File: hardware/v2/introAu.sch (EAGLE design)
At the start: 24 parts

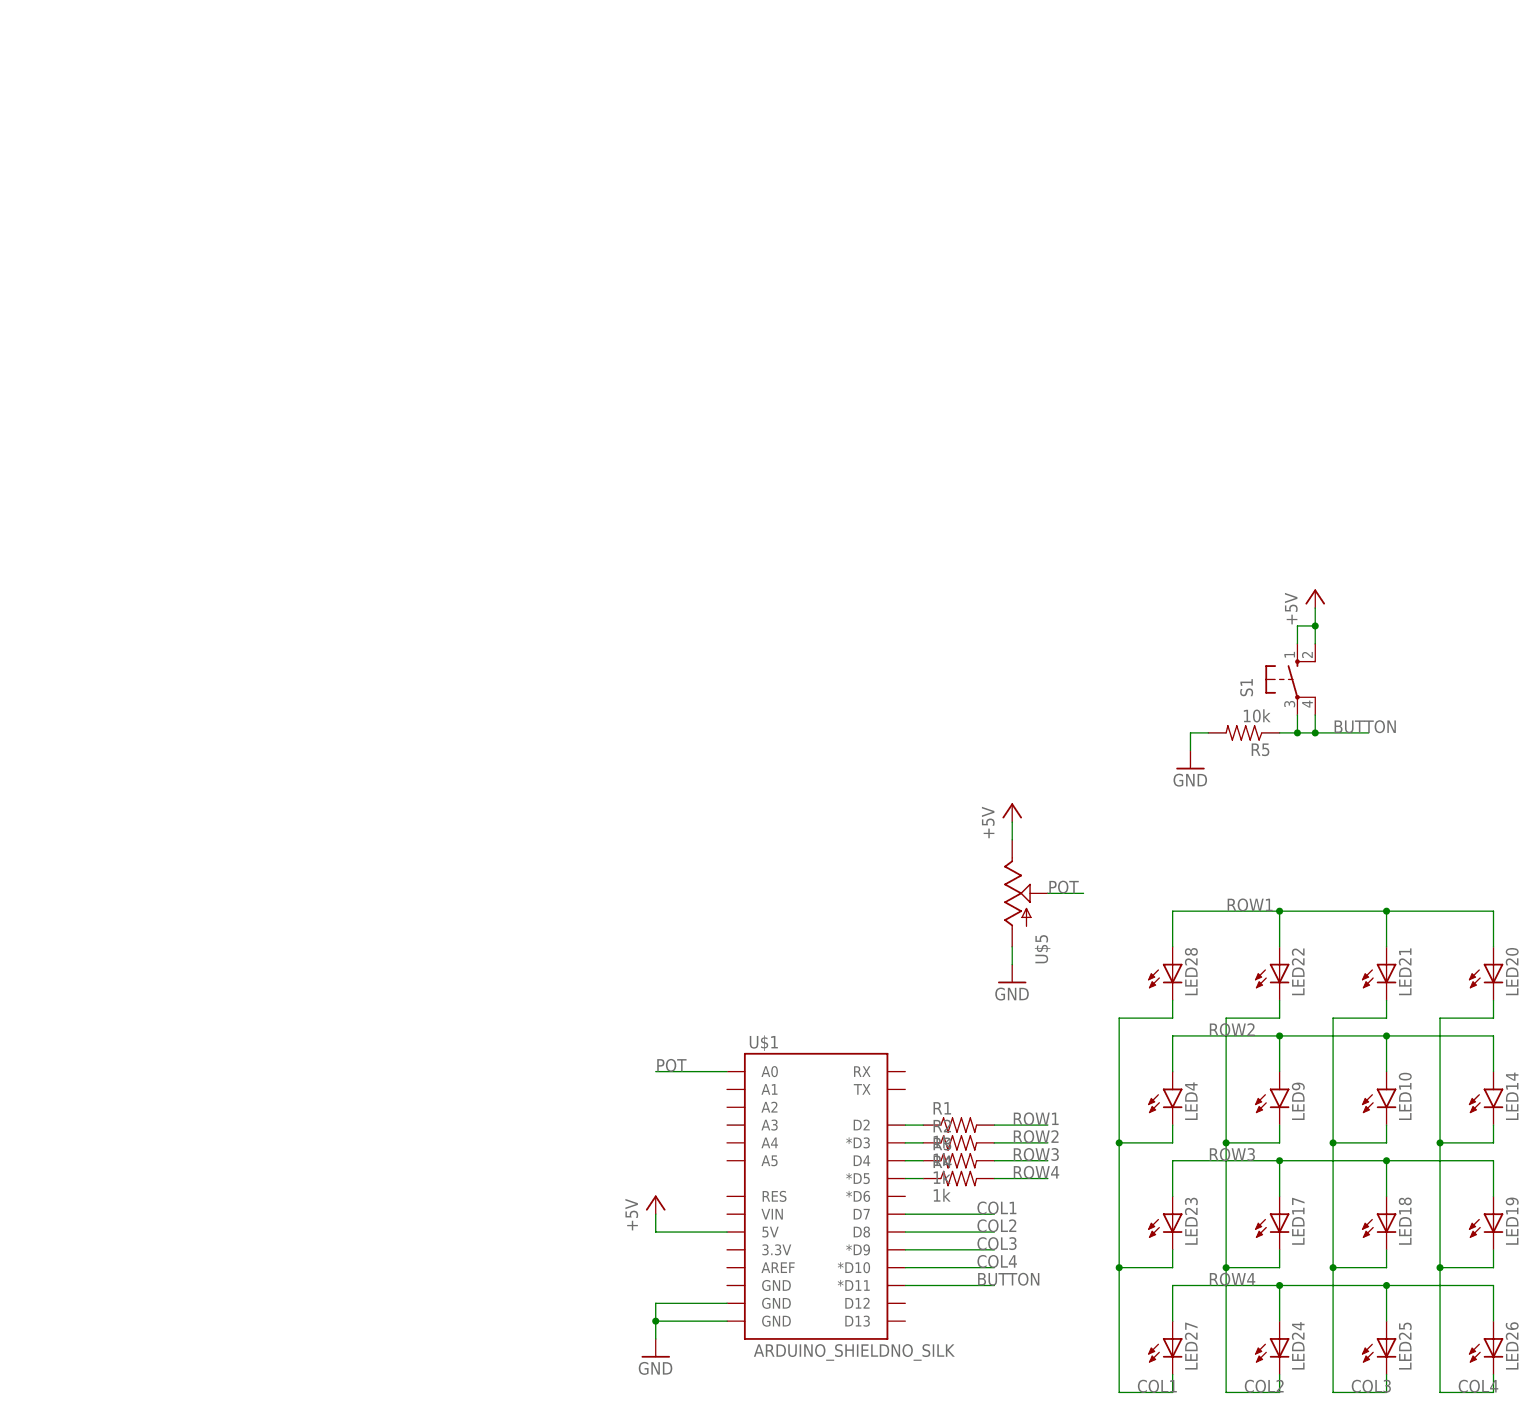
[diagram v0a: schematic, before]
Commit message: Merged in Leonardo onboard
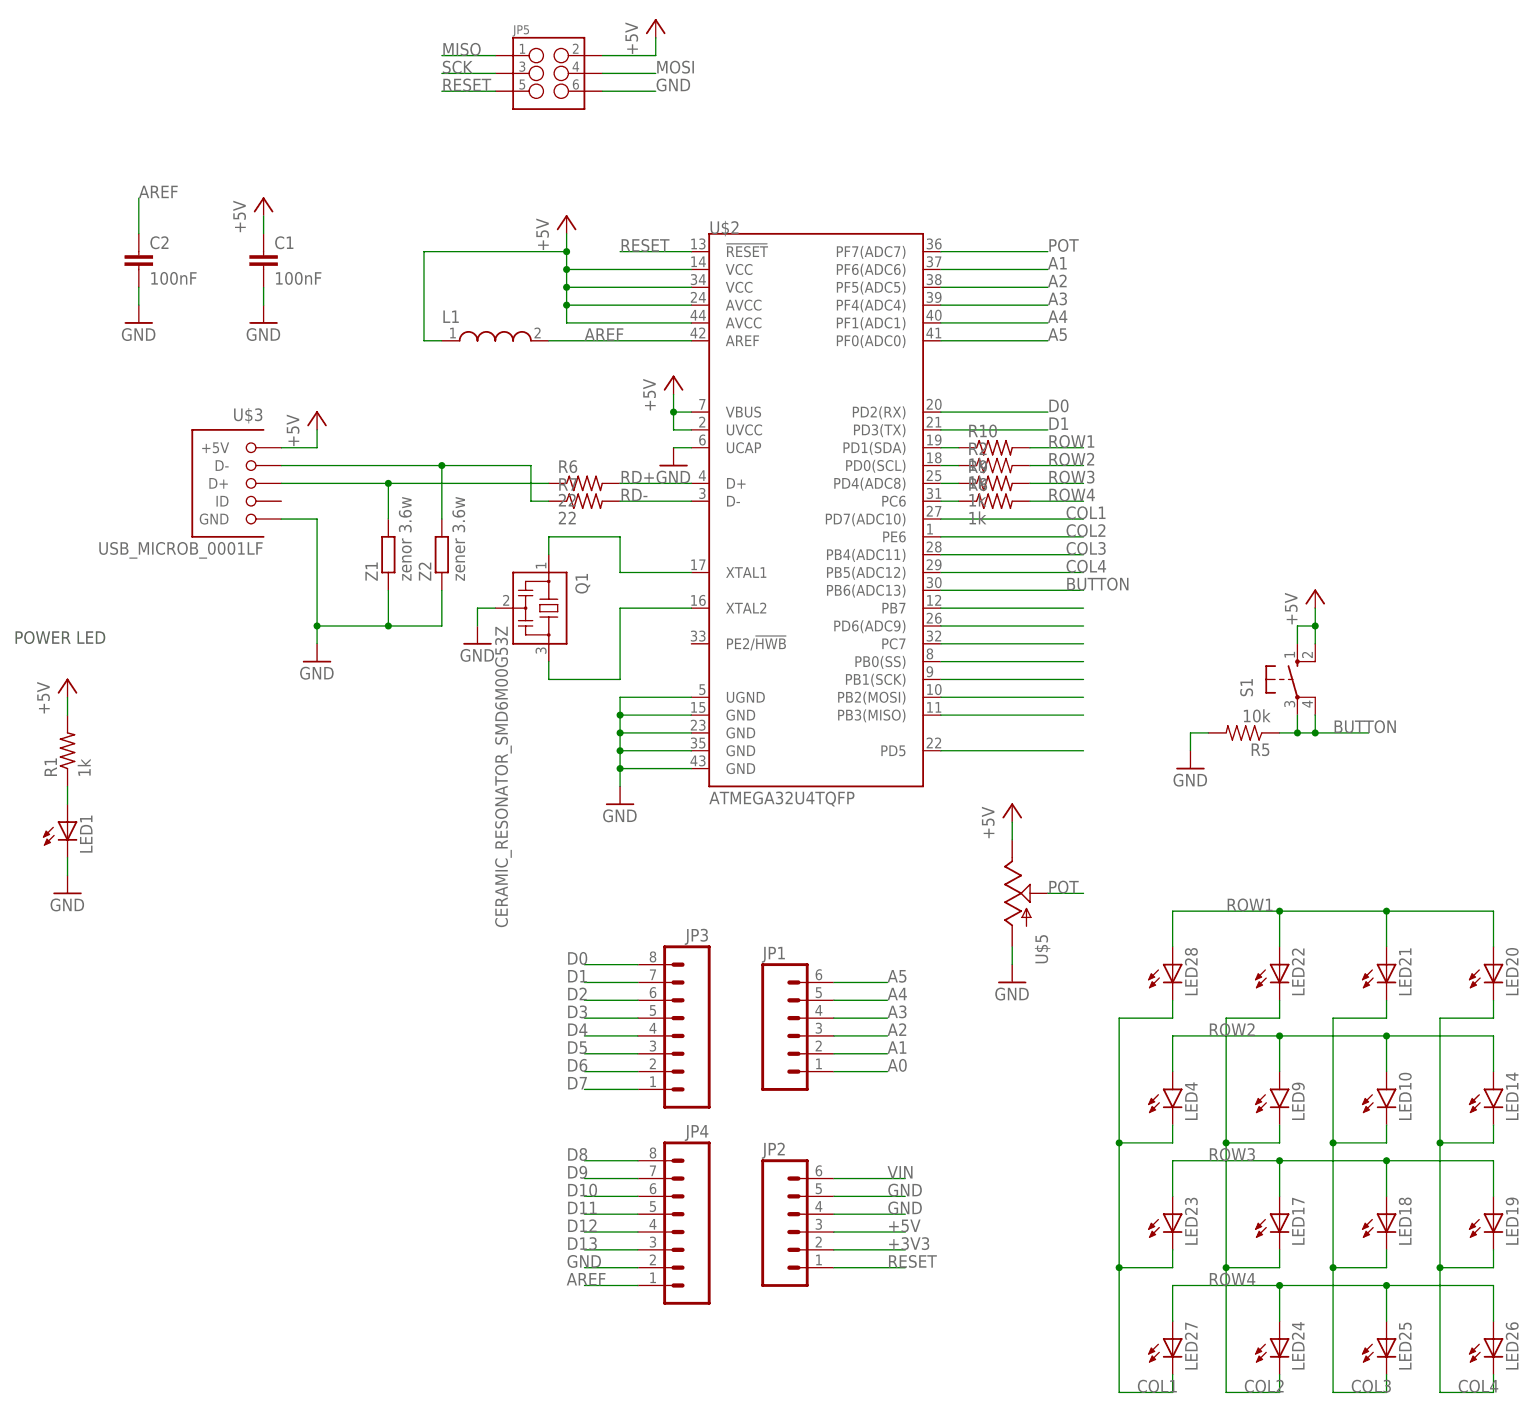
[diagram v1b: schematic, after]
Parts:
- removed R3, R4: 1k, SparkFun-Resistors:1KOHM1/4W5%(PTH)HORIZ-KIT
- removed U$1: ARDUINO_SHIELDNO_SILK, SparkFun-Boards:ARDUINO_SHIELDNO_SILK
- added C1, C2: 100nF, rcl:C-EUC0805
- added JP1, JP2: (no value), SparkFun-Connectors:M06SMD-STRAIGHT-COMBO
- added JP3, JP4: (no value), SparkFun-Connectors:M08SMD-COMBO
- added JP5: (no value), SparkFun-Connectors:M03X22X3_SILK_SM
- added L1: (no value), EagleLibrary_Wuerth_Elektronik_eiSos_rev15c:WE-CBF_0805(WB/HS)
- added LED1: (no value), led:LEDCHIPLED_0805
- added Q1: CERAMIC_RESONATOR_SMD6M00G53Z, MESH_Arduino:CERAMIC_RESONATOR_SMD6M00G53Z
- added R10, R8, R9: 1k, rcl:R-US_R0805
- added R6, R7: 22, rcl:R-US_R0805
- added U$2: ATMEGA32U4TQFP, SparkFun-DigitalIC:ATMEGA32U4TQFP
- added U$3: USB_MICROB_0001LF, mBLE:USB_MICROB_0001LF
- added Z1: zenor 3.6w, rcl:R-EU_R0603
- added Z2: zener 3.6w, rcl:R-EU_R0603
- R1: device SparkFun-Resistors:1KOHM1/4W5%(PTH)HORIZ-KIT -> rcl:R-US_R0805
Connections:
- removed net N$16: R1.1, U$1.D2
- removed net N$17: R2.1, U$1.*D3
- removed net N$18: R3.1, U$1.D4
- removed net N$19: R4.1, U$1.*D5
- new net +3V3: JP2.2
- new net A0: JP1.1
- new net A1: JP1.2, U$2.PF6(ADC6)
- new net A2: JP1.3, U$2.PF5(ADC5)
- new net A3: JP1.4, U$2.PF4(ADC4)
- new net A4: JP1.5, U$2.PF1(ADC1)
- new net A5: JP1.6, U$2.PF0(ADC0)
- new net AREF: C2.1, JP4.1, L1.2, U$2.AREF
- new net D0: JP3.8, U$2.PD2(RX)
- new net D1: JP3.7, U$2.PD3(TX)
- new net D10: JP4.6
- new net D11: JP4.5, U$2.PB7
- new net D12: JP4.4, U$2.PD6(ADC9)
- new net D13: JP4.3, U$2.PC7
- new net D14: U$2.PB3(MISO)
- new net D15: U$2.PB1(SCK)
- new net D16: U$2.PB2(MOSI)
- new net D17: U$2.PB0(SS)
- new net D2: JP3.6
- new net D3: JP3.5
- new net D4: JP3.4
- new net D5: JP3.3
- new net D6: JP3.2
- new net D7: JP3.1
- new net D8: JP4.8
- new net D9: JP4.7
- new net MISO: JP5.1
- new net MOSI: JP5.4
- new net N$1: R10.1, U$2.PD1(SDA)
- new net N$11: LED1.A, R1.1
- new net N$2: R2.1, U$2.PD0(SCL)
- new net N$3: R9.1, U$2.PD4(ADC8)
- new net N$4: R8.1, U$2.PC6
- new net N$5: Q1.3, U$2.XTAL2
- new net N$6: Q1.1, U$2.XTAL1
- new net N$7: R7.1, U$3.D-, Z2.2
- new net N$9: R6.1, U$3.D+, Z1.2
- new net RD+: R6.2, U$2.D+
- new net RD-: R7.2, U$2.D-
- new net RESET: JP2.1, JP5.5, U$2.!RESET
- new net SCK: JP5.3
- new net TX: U$2.PD5
- new net VIN: JP2.6
- net +5V: now also C1.1, JP2.3, JP5.2, L1.1, R1.2, U$2.AVCC@24, U$2.AVCC@44, U$2.UVCC, U$2.VBUS, U$2.VCC@14, U$2.VCC@34, U$3.+5V; no longer U$1.5V
- net BUTTON: now also U$2.PB6(ADC13); no longer U$1.*D11
- net COL1: now also U$2.PD7(ADC10); no longer U$1.D7
- net COL2: now also U$2.PE6; no longer U$1.D8
- net COL3: now also U$2.PB4(ADC11); no longer U$1.*D9
- net COL4: now also U$2.PB5(ADC12); no longer U$1.*D10
- net GND: now also C1.2, C2.2, JP2.4, JP2.5, JP4.2, JP5.6, LED1.C, Q1.2, U$2.GND@15, U$2.GND@23, U$2.GND@35, U$2.GND@43, U$2.UCAP, U$2.UGND, U$3.GND, Z1.1, Z2.1; no longer U$1.GND@0, U$1.GND@1
- net POT: now also U$2.PF7(ADC7); no longer U$1.A0
- net ROW1: now also R10.2; no longer R1.2
- net ROW3: now also R9.2; no longer R3.2
- net ROW4: now also R8.2; no longer R4.2
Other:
- note added: "POWER LED"
- moved on the sheet: R1, R2
